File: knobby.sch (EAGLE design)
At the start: 18 parts

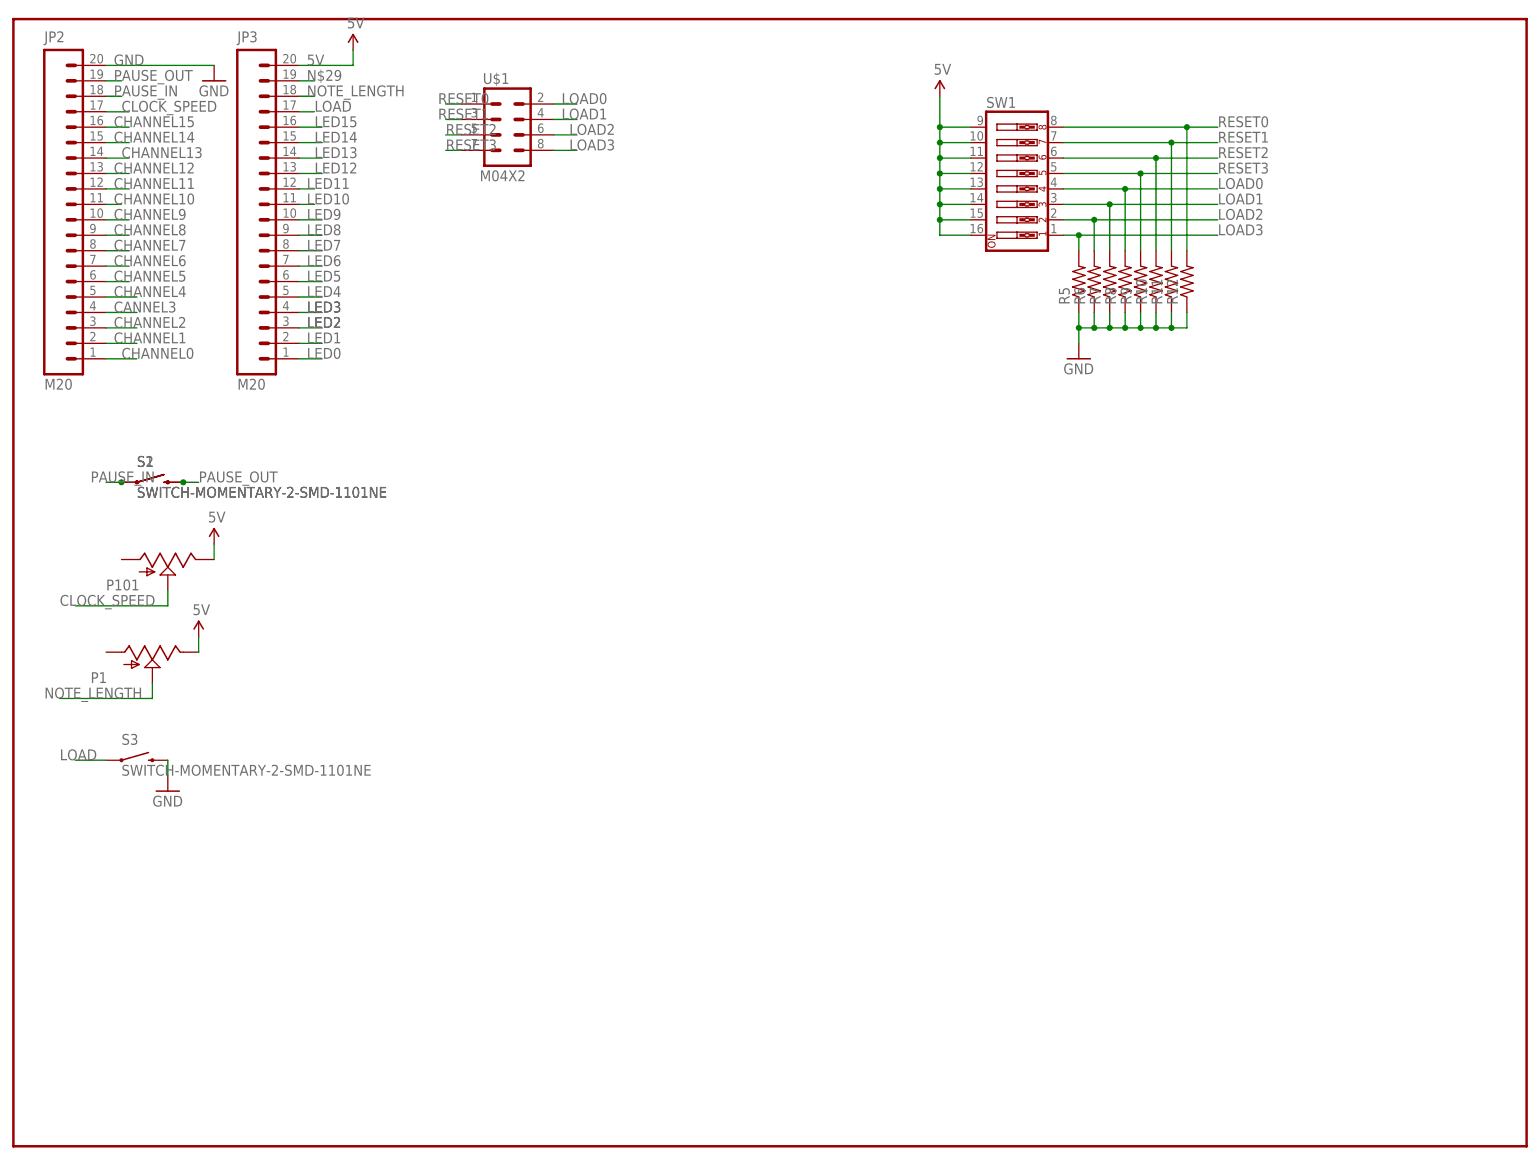
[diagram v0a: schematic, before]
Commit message: 16 pots
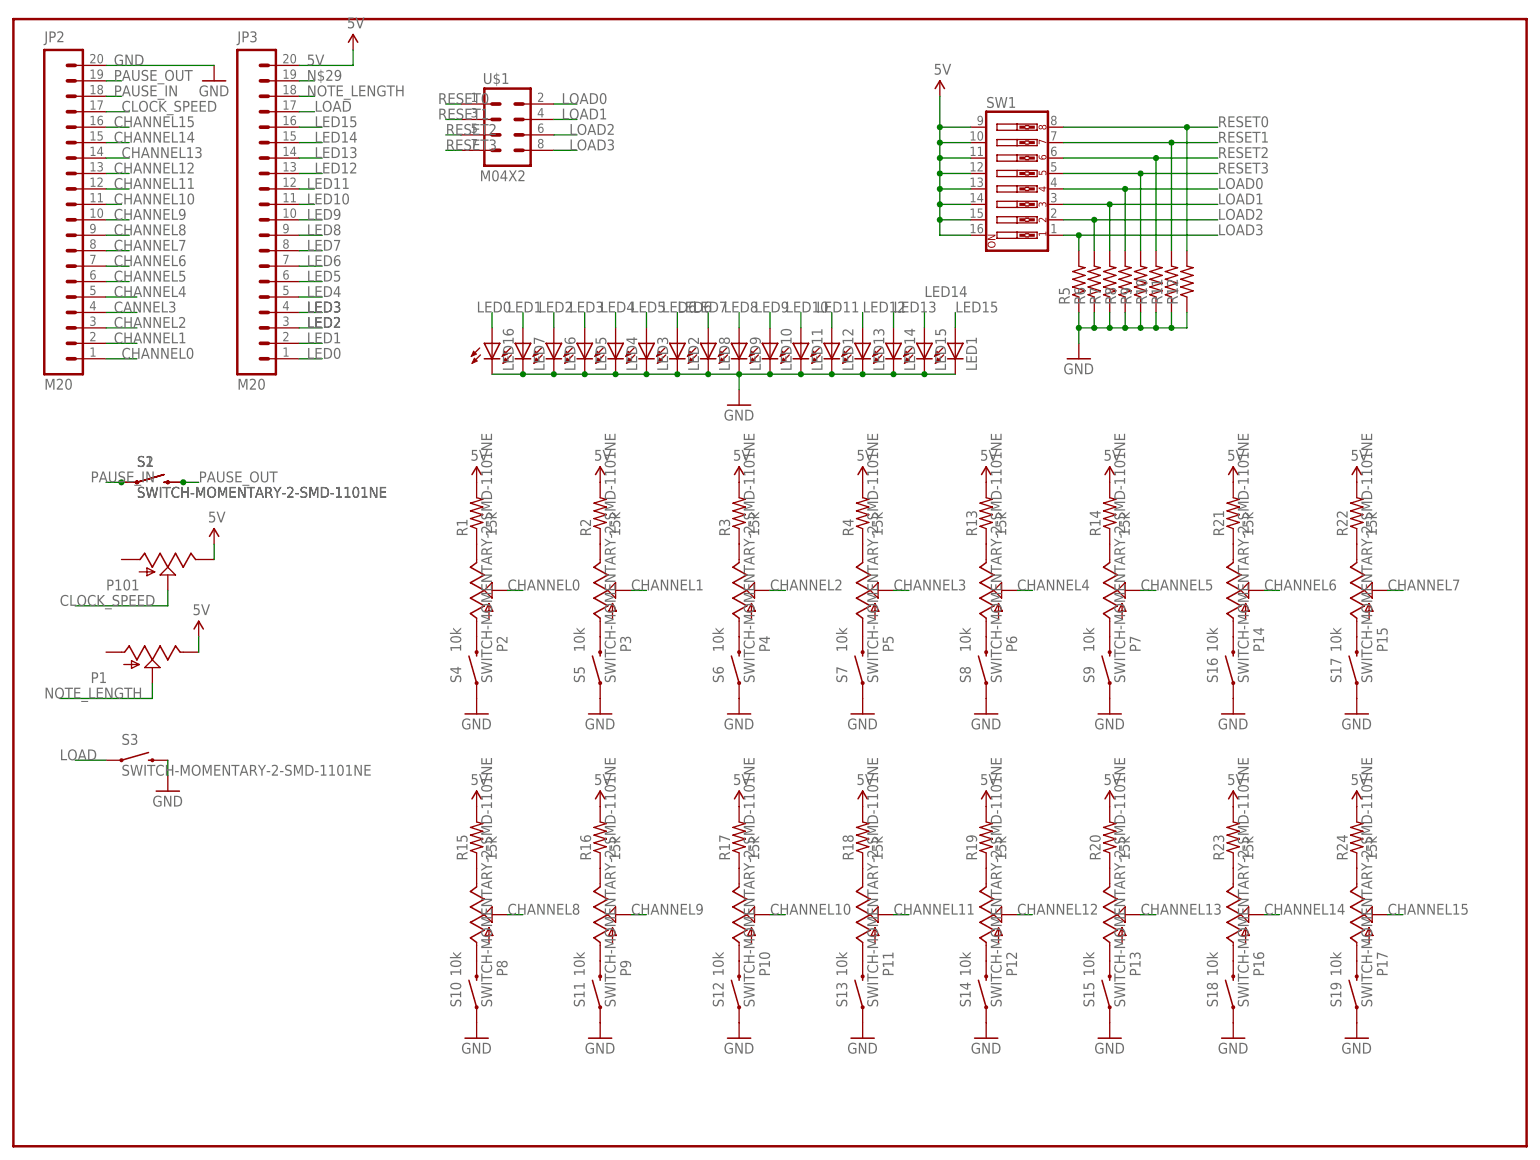
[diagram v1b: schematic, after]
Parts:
- added LED1, LED10, LED11, LED12, LED13, LED14, LED15, LED16, LED2, LED3, LED4, LED5, LED6, LED7, LED8, LED9: (no value), SparkFun-LED:LED0603
- added P10, P11, P12, P13, P14, P15, P16, P17, P2, P3, P4, P5, P6, P7, P8, P9: 10k, DCO_PIGGY:SPARKFUN_POTPDB12
- added R1, R13, R14, R15, R16, R17, R18, R19, R2, R20, R21, R22, R23, R24, R3, R4: 15k, SparkFun-Resistors:RESISTOR0603
- added S10, S11, S12, S13, S14, S15, S16, S17, S18, S19, S4, S5, S6, S7, S8, S9: SWITCH-MOMENTARY-2-SMD-1101NE, SparkFun-Electromechanical:SWITCH-MOMENTARY-2-SMD-1101NE
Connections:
- new net CHANNEL3: P5.S
- new net N$1: P2.E, R1.1
- new net N$10: P6.A, S8.2
- new net N$11: P7.E, R14.1
- new net N$12: P7.A, S9.2
- new net N$13: P8.E, R15.1
- new net N$14: P8.A, S10.2
- new net N$15: P9.E, R16.1
- new net N$16: P9.A, S11.2
- new net N$17: P10.E, R17.1
- new net N$18: P10.A, S12.2
- new net N$19: P11.E, R18.1
- new net N$2: P2.A, S4.2
- new net N$20: P11.A, S13.2
- new net N$21: P12.E, R19.1
- new net N$22: P12.A, S14.2
- new net N$23: P13.E, R20.1
- new net N$24: P13.A, S15.2
- new net N$25: P14.E, R21.1
- new net N$26: P14.A, S16.2
- new net N$27: P15.E, R22.1
- new net N$28: P15.A, S17.2
- new net N$3: P3.E, R2.1
- new net N$30: P16.E, R23.1
- new net N$31: P16.A, S18.2
- new net N$32: P17.E, R24.1
- new net N$33: P17.A, S19.2
- new net N$4: P3.A, S5.2
- new net N$5: P4.E, R3.1
- new net N$6: P4.A, S6.2
- new net N$7: P5.E, R4.1
- new net N$8: P5.A, S7.2
- new net N$9: P6.E, R13.1
- net 5V: now also R1.2, R13.2, R14.2, R15.2, R16.2, R17.2, R18.2, R19.2, R2.2, R20.2, R21.2, R22.2, R23.2, R24.2, R3.2, R4.2
- net CHANNEL0: now also P2.S
- net CHANNEL1: now also P3.S
- net CHANNEL10: now also P10.S
- net CHANNEL11: now also P11.S
- net CHANNEL12: now also P12.S
- net CHANNEL13: now also P13.S
- net CHANNEL14: now also P16.S
- net CHANNEL15: now also P17.S
- net CHANNEL2: now also P4.S
- net CHANNEL4: now also P6.S
- net CHANNEL5: now also P7.S
- net CHANNEL6: now also P14.S
- net CHANNEL7: now also P15.S
- net CHANNEL8: now also P8.S
- net CHANNEL9: now also P9.S
- net GND: now also LED1.C, LED10.C, LED11.C, LED12.C, LED13.C, LED14.C, LED15.C, LED16.C, LED2.C, LED3.C, LED4.C, LED5.C, LED6.C, LED7.C, LED8.C, LED9.C, S10.1, S11.1, S12.1, S13.1, S14.1, S15.1, S16.1, S17.1, S18.1, S19.1, S4.1, S5.1, S6.1, S7.1, S8.1, S9.1
- net LED0: now also LED16.A
- net LED1: now also LED7.A
- net LED10: now also LED11.A
- net LED11: now also LED12.A
- net LED12: now also LED13.A
- net LED13: now also LED14.A
- net LED14: now also LED15.A
- net LED15: now also LED1.A
- net LED2: now also LED6.A
- net LED3: now also LED5.A
- net LED4: now also LED4.A
- net LED5: now also LED3.A
- net LED6: now also LED2.A
- net LED7: now also LED8.A
- net LED8: now also LED9.A
- net LED9: now also LED10.A

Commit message: knobby brd
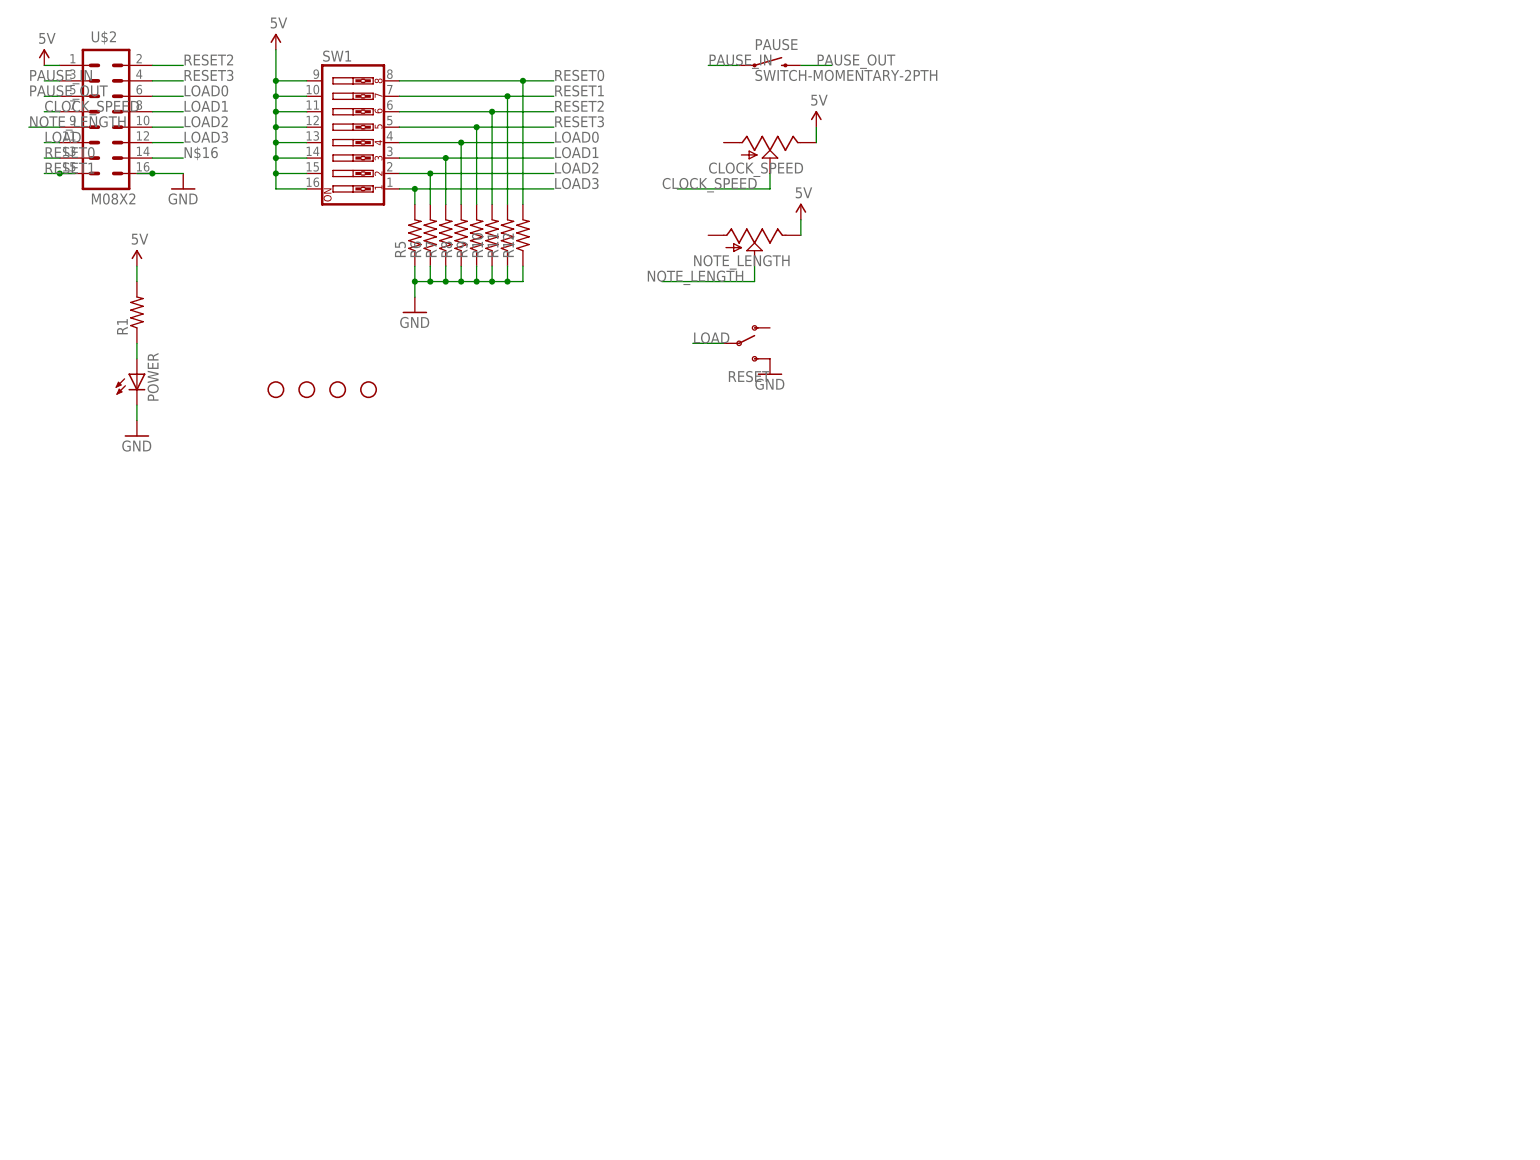
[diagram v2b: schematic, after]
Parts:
- removed FRAME1: FRAME-LETTER, SparkFun-Aesthetics:FRAME-LETTER
- removed JP2, JP3: M20, SparkFun-Connectors:M20
- removed LED1, LED10, LED11, LED12, LED13, LED14, LED15, LED16, LED2, LED3, LED4, LED5, LED6, LED7, LED8, LED9: (no value), SparkFun-LED:LED0603
- removed P1, P101: (no value), DCO_PIGGY:SPARKFUN_POTPDB12
- removed P10, P11, P12, P13, P14, P15, P16, P17, P2, P3, P4, P5, P6, P7, P8, P9: 10k, DCO_PIGGY:SPARKFUN_POTPDB12
- removed R13, R14, R15, R16, R17, R18, R19, R2, R20, R21, R22, R23, R24, R3, R4: 15k, SparkFun-Resistors:RESISTOR0603
- removed S1, S10, S11, S12, S13, S14, S15, S16, S17, S18, S19, S2, S3, S4, S5, S6, S7, S8, S9: SWITCH-MOMENTARY-2-SMD-1101NE, SparkFun-Electromechanical:SWITCH-MOMENTARY-2-SMD-1101NE
- removed U$1: M04X2, SparkFun-Connectors:M04X2
- added CLOCK_SPEED, NOTE_LENGTH: (no value), DCO_PIGGY:SPARKFUN_POTPDB12
- added PAUSE: SWITCH-MOMENTARY-2PTH, SparkFun-Electromechanical:SWITCH-MOMENTARY-2PTH
- added POWER: (no value), SparkFun-LED:LED3MM
- added RESET: (no value), SparkFun-Electromechanical:SWITCH-SPDTPTH
- added STANDOFF1, STANDOFF2, STANDOFF3, STANDOFF4: STAND-OFF, SparkFun-Electromechanical:STAND-OFF
- added U$2: M08X2, SparkFun-Connectors:M08X2
- R1: value 15k -> (none)
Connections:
- removed net CANNEL3: JP2.4
- removed net CHANNEL0: JP2.1, P2.S
- removed net CHANNEL1: JP2.2, P3.S
- removed net CHANNEL10: JP2.11, P10.S
- removed net CHANNEL11: JP2.12, P11.S
- removed net CHANNEL12: JP2.13, P12.S
- removed net CHANNEL13: JP2.14, P13.S
- removed net CHANNEL14: JP2.15, P16.S
- removed net CHANNEL15: JP2.16, P17.S
- removed net CHANNEL2: JP2.3, P4.S
- removed net CHANNEL3: P5.S
- removed net CHANNEL4: JP2.5, P6.S
- removed net CHANNEL5: JP2.6, P7.S
- removed net CHANNEL6: JP2.7, P14.S
- removed net CHANNEL7: JP2.8, P15.S
- removed net CHANNEL8: JP2.9, P8.S
- removed net CHANNEL9: JP2.10, P9.S
- removed net LED0: JP3.1, LED16.A
- removed net LED1: JP3.2, LED7.A
- removed net LED10: JP3.11, LED11.A
- removed net LED11: JP3.12, LED12.A
- removed net LED12: JP3.13, LED13.A
- removed net LED13: JP3.14, LED14.A
- removed net LED14: JP3.15, LED15.A
- removed net LED15: JP3.16, LED1.A
- removed net LED2: JP3.3, LED6.A
- removed net LED3: JP3.4, LED5.A
- removed net LED4: JP3.5, LED4.A
- removed net LED5: JP3.6, LED3.A
- removed net LED6: JP3.7, LED2.A
- removed net LED7: JP3.8, LED8.A
- removed net LED8: JP3.9, LED9.A
- removed net LED9: JP3.10, LED10.A
- removed net N$10: P6.A, S8.2
- removed net N$11: P7.E, R14.1
- removed net N$12: P7.A, S9.2
- removed net N$13: P8.E, R15.1
- removed net N$14: P8.A, S10.2
- removed net N$15: P9.E, R16.1
- removed net N$17: P10.E, R17.1
- removed net N$18: P10.A, S12.2
- removed net N$19: P11.E, R18.1
- removed net N$2: P2.A, S4.2
- removed net N$20: P11.A, S13.2
- removed net N$21: P12.E, R19.1
- removed net N$22: P12.A, S14.2
- removed net N$23: P13.E, R20.1
- removed net N$24: P13.A, S15.2
- removed net N$25: P14.E, R21.1
- removed net N$26: P14.A, S16.2
- removed net N$27: P15.E, R22.1
- removed net N$28: P15.A, S17.2
- removed net N$29: JP3.19
- removed net N$3: P3.E, R2.1
- removed net N$30: P16.E, R23.1
- removed net N$31: P16.A, S18.2
- removed net N$32: P17.E, R24.1
- removed net N$33: P17.A, S19.2
- removed net N$4: P3.A, S5.2
- removed net N$5: P4.E, R3.1
- removed net N$6: P4.A, S6.2
- removed net N$7: P5.E, R4.1
- removed net N$8: P5.A, S7.2
- removed net N$9: P6.E, R13.1
- net 5V: now also CLOCK_SPEED.E, NOTE_LENGTH.E, U$2.1; no longer JP3.20, P1.E, P101.E, R13.2, R14.2, R15.2, R16.2, R17.2, R18.2, R19.2, R2.2, R20.2, R21.2, R22.2, R23.2, R24.2, R3.2, R4.2
- net CLOCK_SPEED: now also CLOCK_SPEED.S, U$2.7; no longer JP2.17, P101.S
- net GND: now also POWER.C, RESET.S, U$2.16; no longer JP2.20, LED1.C, LED10.C, LED11.C, LED12.C, LED13.C, LED14.C, LED15.C, LED16.C, LED2.C, LED3.C, LED4.C, LED5.C, LED6.C, LED7.C, LED8.C, LED9.C, S10.1, S11.1, S12.1, S13.1, S14.1, S15.1, S16.1, S17.1, S18.1, S19.1, S3.2, S4.1, S5.1, S6.1, S7.1, S8.1, S9.1
- net LOAD: now also RESET.P, U$2.11; no longer JP3.17, S3.1
- net LOAD0: now also U$2.6; no longer U$1.2
- net LOAD1: now also U$2.8; no longer U$1.4
- net LOAD2: now also U$2.10; no longer U$1.6
- net LOAD3: now also U$2.12; no longer U$1.8
- net N$1: now also POWER.A; no longer P2.E
- net N$16: now also U$2.14; no longer P9.A, S11.2
- net NOTE_LENGTH: now also NOTE_LENGTH.S, U$2.9; no longer JP3.18, P1.S
- net PAUSE_IN: now also PAUSE.1, U$2.3; no longer JP2.18, S1.1, S2.1
- net PAUSE_OUT: now also PAUSE.2, U$2.5; no longer JP2.19, S1.2, S2.2
- net RESET0: now also U$2.13; no longer U$1.1
- net RESET1: now also U$2.15; no longer U$1.3
- net RESET2: now also U$2.2; no longer U$1.5
- net RESET3: now also U$2.4; no longer U$1.7
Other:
- moved on the sheet: R1, R10, R11, R12, R5, R6, R7, R8, R9, SW1
